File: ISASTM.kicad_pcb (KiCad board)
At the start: 2 copper layers, 1 part, among them J1 Bus_ISA_16bit

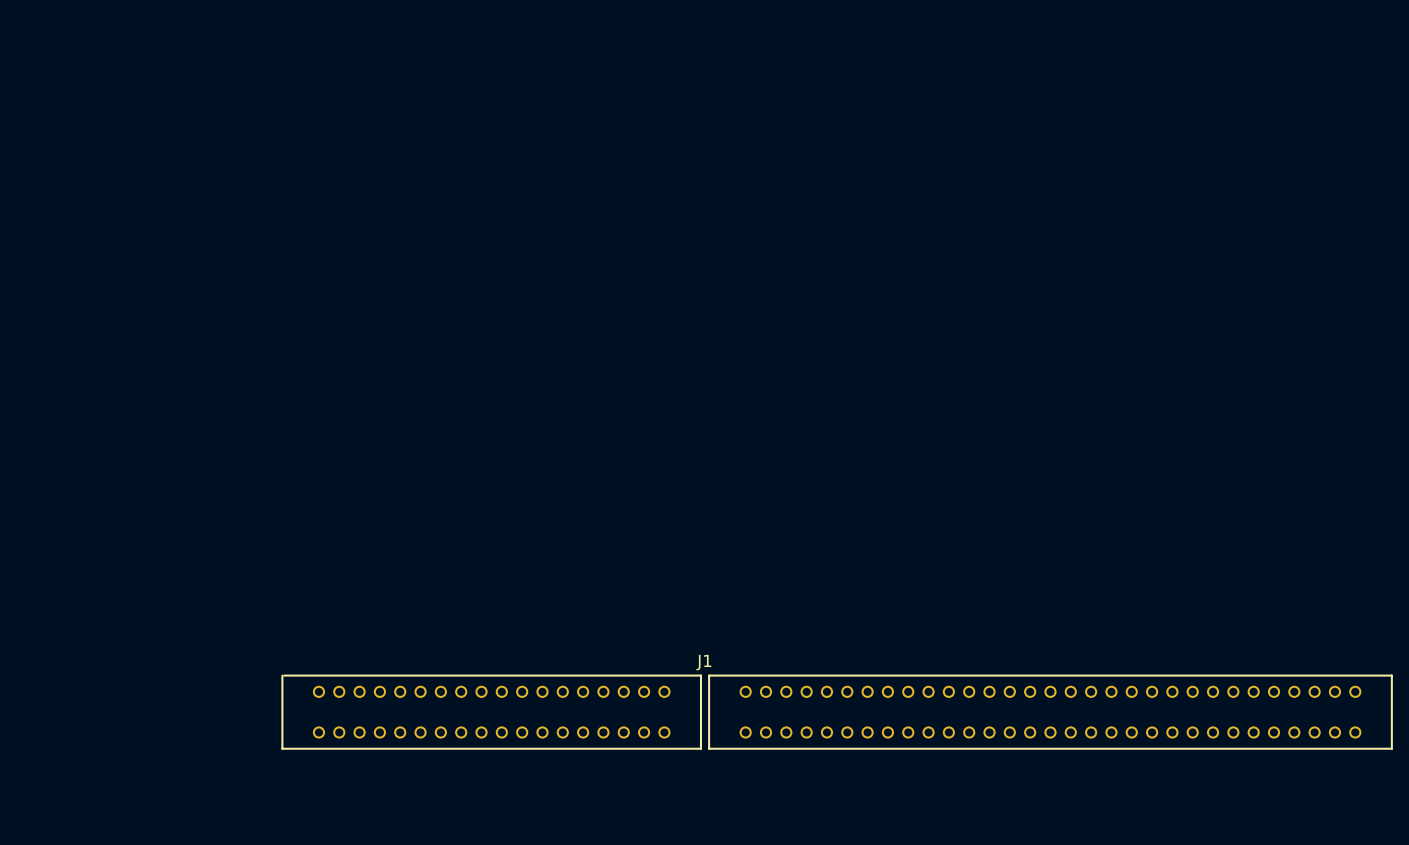
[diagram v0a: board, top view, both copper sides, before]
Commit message: Add connector
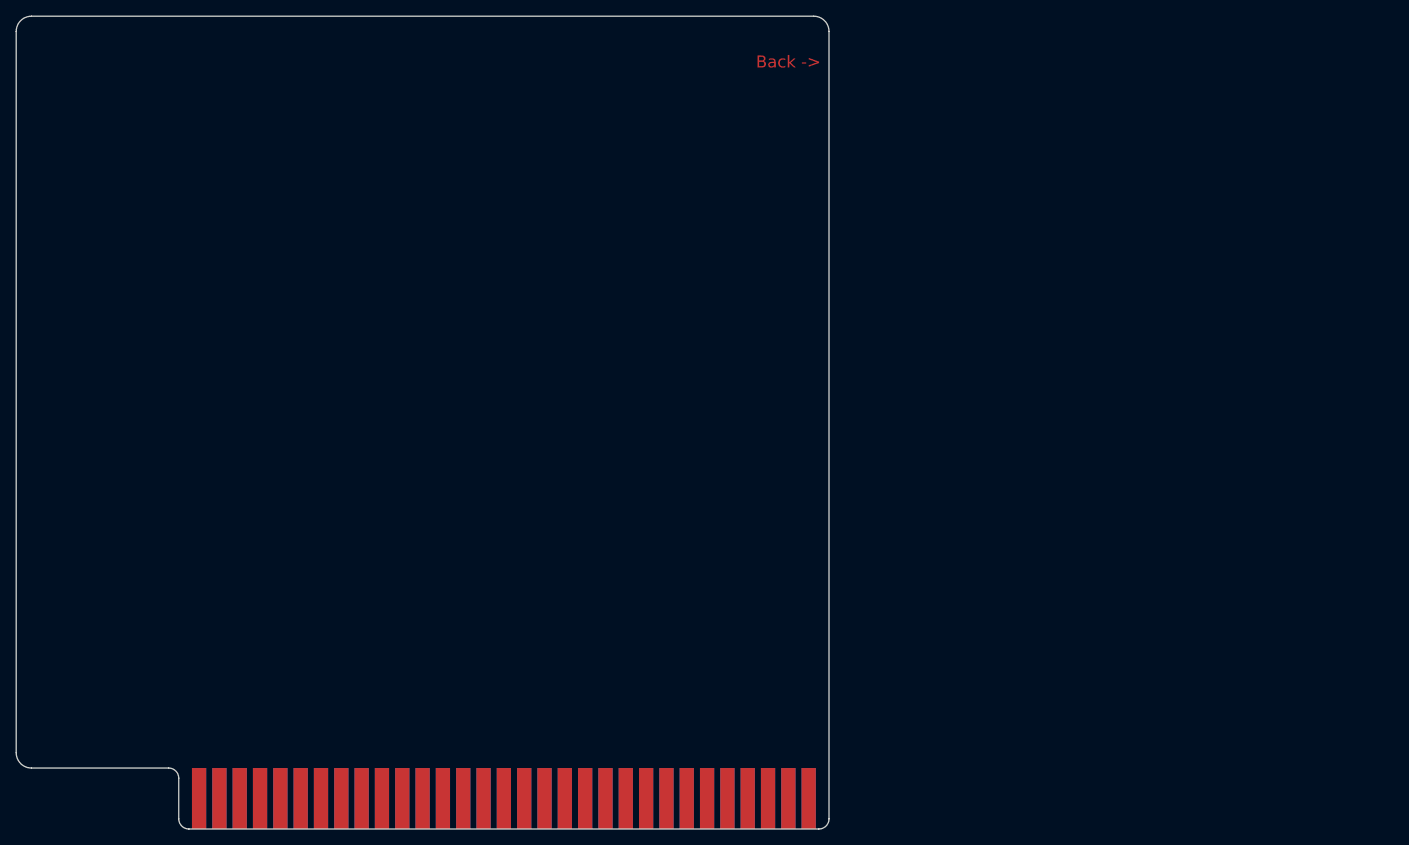
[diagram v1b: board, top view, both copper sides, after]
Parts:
- J1: value Bus_ISA_16bit -> Bus_ISA_8bit; footprint isastm:ISA16 -> ISASTM:Conn_Edge_PCB_ISA8
- moved J1 43.0 mm to (76.2, 112.4)
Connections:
- net Net-(J1-Pad11) renamed /~SMEMW
- net Net-(J1-Pad12) renamed /~SMEMR
- net Net-(J1-Pad13) renamed /~IOW
- net Net-(J1-Pad14) renamed /~IOR
- net Net-(J1-Pad15) renamed /~DACK3
- net Net-(J1-Pad16) renamed /DRQ3
- net Net-(J1-Pad17) renamed /~DACK1
- net Net-(J1-Pad18) renamed /DRQ1
- net Net-(J1-Pad19) renamed /~REFRESH
- net Net-(J1-Pad2) renamed /RESET
- net Net-(J1-Pad20) renamed /CLK
- net Net-(J1-Pad21) renamed /IRQ7
- net Net-(J1-Pad22) renamed /IRQ6
- net Net-(J1-Pad23) renamed /IRQ5
- net Net-(J1-Pad24) renamed /IRQ4
- net Net-(J1-Pad25) renamed /IRQ3
- net Net-(J1-Pad26) renamed /~DACK2
- net Net-(J1-Pad27) renamed /TC
- net Net-(J1-Pad28) renamed /ALE
- net Net-(J1-Pad30) renamed /OSC
- net Net-(J1-Pad32) renamed /~IO_CH_CK
- net Net-(J1-Pad33) renamed /D7
- net Net-(J1-Pad34) renamed /D6
- net Net-(J1-Pad35) renamed /D5
- net Net-(J1-Pad36) renamed /D4
- net Net-(J1-Pad37) renamed /D3
- net Net-(J1-Pad38) renamed /D2
- net Net-(J1-Pad39) renamed /D1
- net Net-(J1-Pad4) renamed /IRQ2
- net Net-(J1-Pad40) renamed /D0
- net Net-(J1-Pad41) renamed /IO_CH_RDY
- net Net-(J1-Pad42) renamed /AEN
- net Net-(J1-Pad43) renamed /A19
- net Net-(J1-Pad44) renamed /A18
- net Net-(J1-Pad45) renamed /A17
- net Net-(J1-Pad46) renamed /A16
- net Net-(J1-Pad47) renamed /A15
- net Net-(J1-Pad48) renamed /A14
- net Net-(J1-Pad49) renamed /A13
- net Net-(J1-Pad5) renamed -5V
- net Net-(J1-Pad50) renamed /A12
- net Net-(J1-Pad51) renamed /A11
- net Net-(J1-Pad52) renamed /A10
- net Net-(J1-Pad53) renamed /A9
- net Net-(J1-Pad54) renamed /A8
- net Net-(J1-Pad55) renamed /A7
- net Net-(J1-Pad56) renamed /A6
- net Net-(J1-Pad57) renamed /A5
- net Net-(J1-Pad58) renamed /A4
- net Net-(J1-Pad59) renamed /A3
- net Net-(J1-Pad6) renamed /DRQ2
- net Net-(J1-Pad60) renamed /A2
- net Net-(J1-Pad61) renamed /A1
- net Net-(J1-Pad62) renamed /A0
- net Net-(J1-Pad7) renamed -12V
- net Net-(J1-Pad9) renamed +12V
- J1 pad 29: Net-(J1-Pad29) -> +5V
- J1 pad 3: Net-(J1-Pad3) -> +5V
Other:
- board outline added: 101.6 x 101.6 mm
- copper layers 2 -> 4
- board text added: "Back ->"
